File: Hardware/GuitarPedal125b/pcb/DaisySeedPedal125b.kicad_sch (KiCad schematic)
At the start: 6 parts, among them J1 Barrel_Jack_Switch, J2 AUDIO_IN_TRS, J3 AUDIO_OUT_TRS, J4 MIDI IN JACK, J5 MIDI OUT JACK

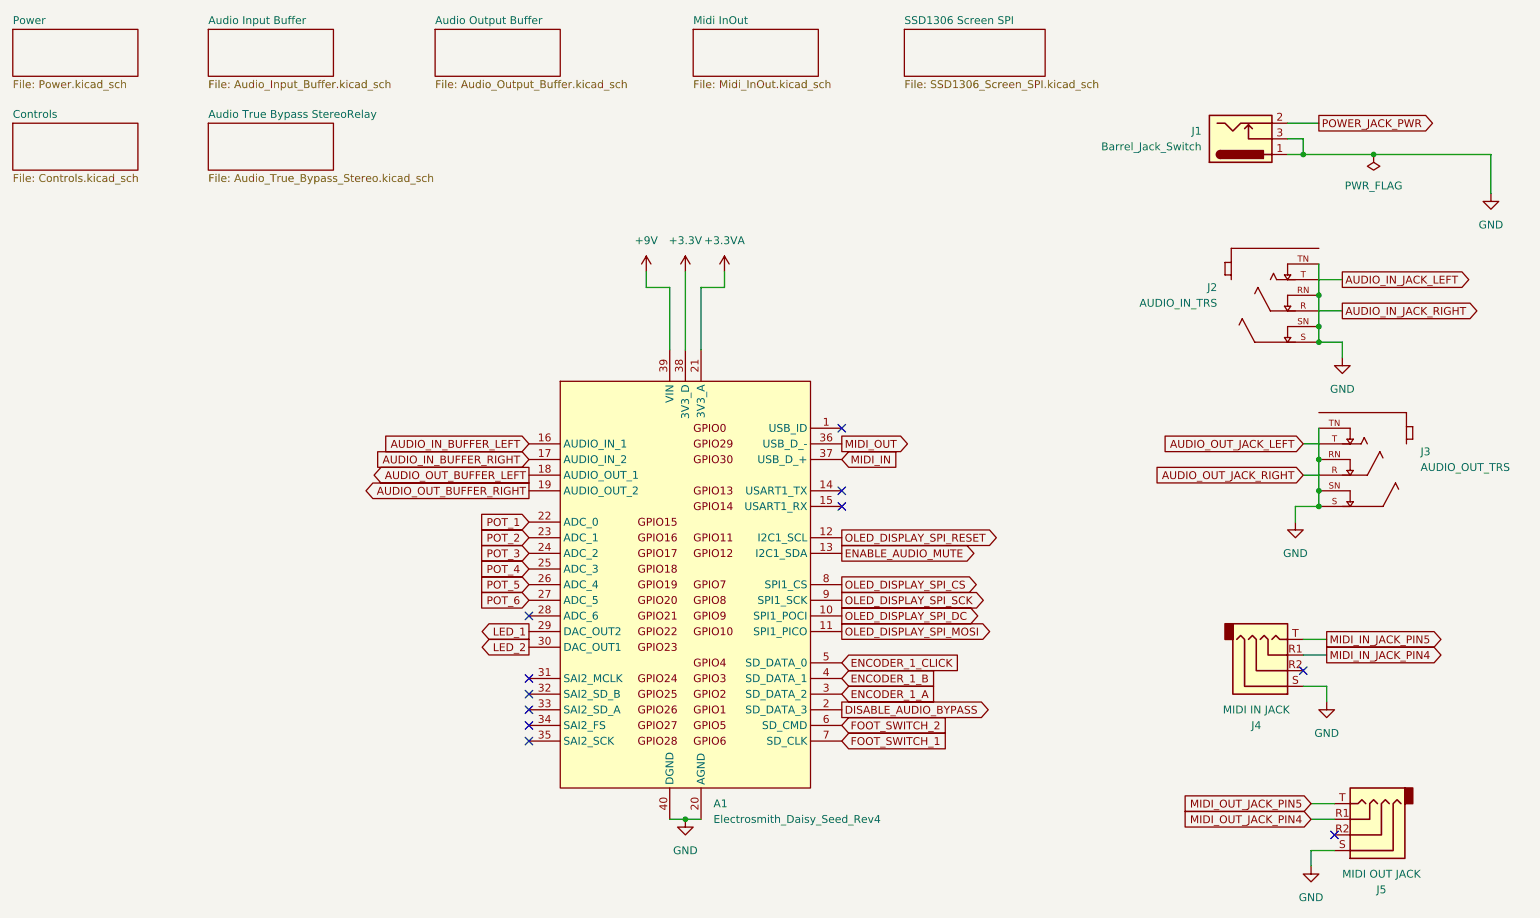
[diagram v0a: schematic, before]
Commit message: Rev6 WIP
Working on a fresh layout of the board.
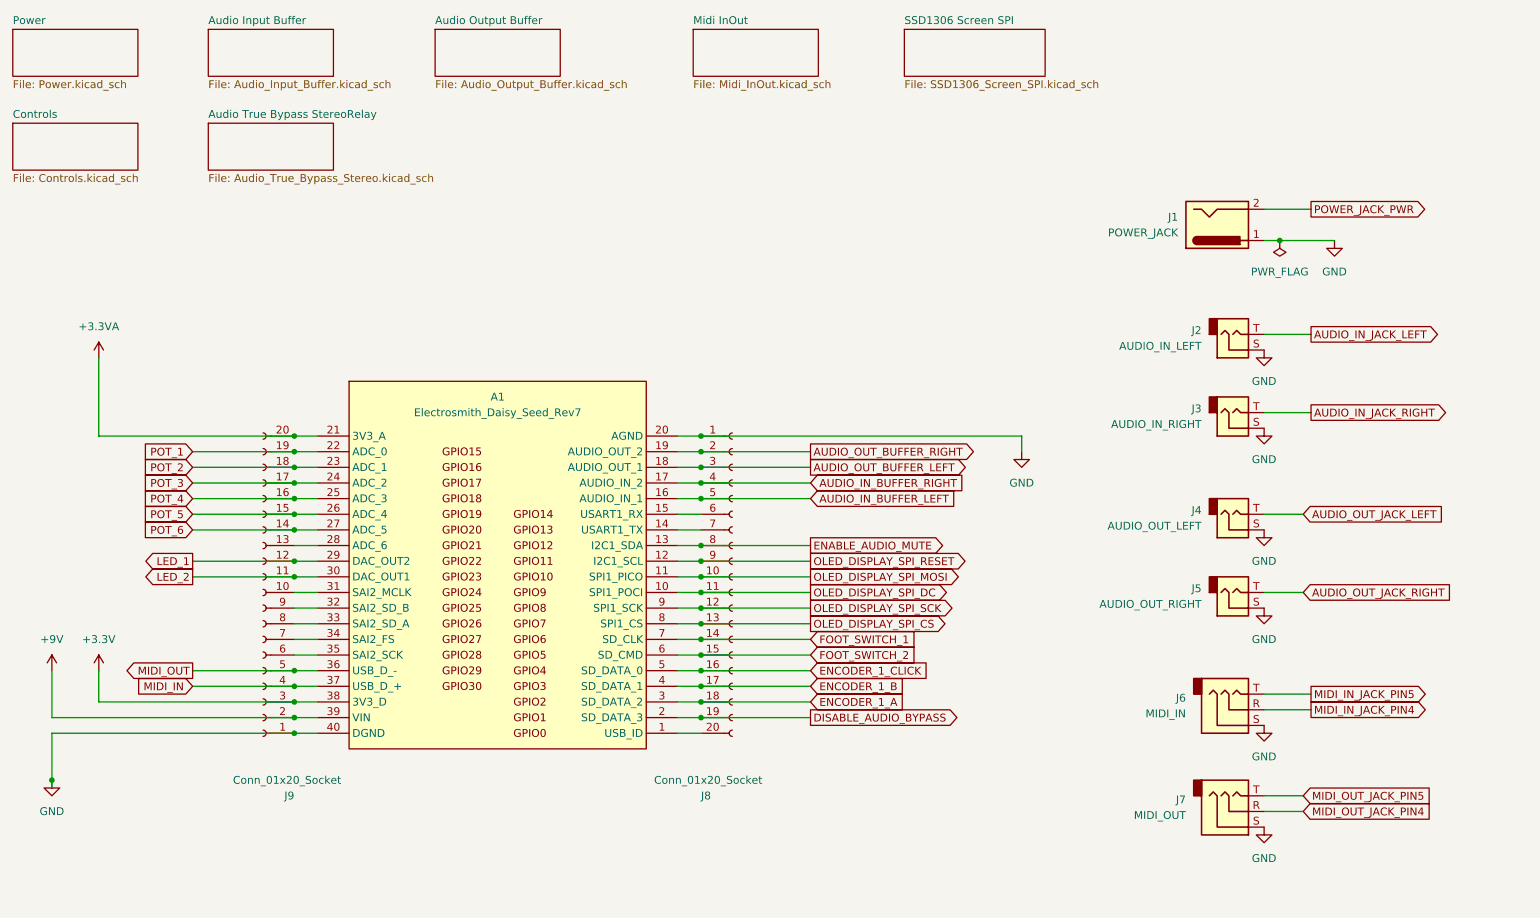
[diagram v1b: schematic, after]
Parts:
- removed J3: AUDIO_OUT_TRS, NMJ6HCD2:NEUTRIK_NMJ6HCD2, symbol NMJ6HCD2:NMJ6HCD2
- removed J5: MIDI OUT JACK, AudioConnector-PJ320A:TRRS-PJ-320A, symbol Connector_Audio:AudioJack4
- added J3: AUDIO_IN_RIGHT, GuitarPedal125B:Generic_Pads_AudioTS, symbol Connector_Audio:AudioJack2
- added J4: AUDIO_OUT_LEFT, GuitarPedal125B:Generic_Pads_AudioTS, symbol Connector_Audio:AudioJack2
- added J5: AUDIO_OUT_RIGHT, GuitarPedal125B:Generic_Pads_AudioTS, symbol Connector_Audio:AudioJack2
- added J7: MIDI_OUT, GuitarPedal125B:Generic_Pads_AudioTRS, symbol Connector_Audio:AudioJack3
- added J8, J9: Conn_01x20_Socket, Connector_PinSocket_2.54mm:PinSocket_1x20_P2.54mm_Vertical, symbol Connector:Conn_01x20_Socket
- A1: value Electrosmith_Daisy_Seed_Rev4 -> Electrosmith_Daisy_Seed_Rev7; footprint Module:Electrosmith_Daisy_Seed -> (none); symbol MCU_Module:Electrosmith_Daisy_Seed_Rev4 -> GuitarPedal125B:Electrosmith_Daisy_Seed_Rev7; now left out of the parts list
- J1: value Barrel_Jack_Switch -> POWER_JACK; footprint GuitarPedal125B:Generic_PowerJack -> GuitarPedal125B:Generic_Pads_Power; symbol Connector:Barrel_Jack_Switch -> Connector:Barrel_Jack
- J2: value AUDIO_IN_TRS -> AUDIO_IN_LEFT; footprint NMJ6HCD2:NEUTRIK_NMJ6HCD2 -> GuitarPedal125B:Generic_Pads_AudioTS; symbol NMJ6HCD2:NMJ6HCD2 -> Connector_Audio:AudioJack2
- J6: renamed from J4; value MIDI IN JACK -> MIDI_IN; footprint AudioConnector-PJ320A:TRRS-PJ-320A -> GuitarPedal125B:Generic_Pads_AudioTRS; symbol Connector_Audio:AudioJack4 -> Connector_Audio:AudioJack3
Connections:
- net +3.3V: now also J9.3 (Pin_3)
- net +3.3VA: now also J9.20 (Pin_20)
- net +9V: now also J9.2 (Pin_2)
- net AUDIO_IN_BUFFER_LEFT: now also J8.5 (Pin_5)
- net AUDIO_IN_BUFFER_RIGHT: now also J8.4 (Pin_4)
- net AUDIO_IN_JACK_RIGHT: now also J3.T; no longer J2.R
- net AUDIO_OUT_BUFFER_LEFT: now also J8.3 (Pin_3)
- net AUDIO_OUT_BUFFER_RIGHT: now also J8.2 (Pin_2)
- net AUDIO_OUT_JACK_LEFT: now also J4.T
- net AUDIO_OUT_JACK_RIGHT: now also J5.T
- net DISABLE_AUDIO_BYPASS: now also J8.19 (Pin_19)
- net ENABLE_AUDIO_MUTE: now also J8.8 (Pin_8)
- net ENCODER_1_A: now also J8.18 (Pin_18)
- net ENCODER_1_B: now also J8.17 (Pin_17)
- net ENCODER_1_CLICK: now also J8.16 (Pin_16)
- net FOOT_SWITCH_1: now also J8.14 (Pin_14)
- net FOOT_SWITCH_2: now also J8.15 (Pin_15)
- net GND: now also J3.S, J4.S, J5.S, J7.S, J8.1 (Pin_1), J9.1 (Pin_1); no longer J1.3, J2.RN, J2.SN, J2.TN
- net LED_1: now also J9.12 (Pin_12)
- net LED_2: now also J9.11 (Pin_11)
- net MIDI_IN: now also J9.4 (Pin_4)
- net MIDI_IN_JACK_PIN4: now also J6.R; no longer J6.R1
- net MIDI_OUT: now also J9.5 (Pin_5)
- net MIDI_OUT_JACK_PIN4: now also J7.R
- net MIDI_OUT_JACK_PIN5: now also J7.T
- net OLED_DISPLAY_SPI_CS: now also J8.13 (Pin_13)
- net OLED_DISPLAY_SPI_DC: now also J8.11 (Pin_11)
- net OLED_DISPLAY_SPI_MOSI: now also J8.10 (Pin_10)
- net OLED_DISPLAY_SPI_RESET: now also J8.9 (Pin_9)
- net OLED_DISPLAY_SPI_SCK: now also J8.12 (Pin_12)
- net POT_1: now also J9.19 (Pin_19)
- net POT_2: now also J9.18 (Pin_18)
- net POT_3: now also J9.17 (Pin_17)
- net POT_4: now also J9.16 (Pin_16)
- net POT_5: now also J9.15 (Pin_15)
- net POT_6: now also J9.14 (Pin_14)
- net at A1.1 (USB_ID): now also J8.20 (Pin_20)
- net at A1.14 (USART1_TX): now also J8.7 (Pin_7)
- net at A1.15 (USART1_RX): now also J8.6 (Pin_6)
- net at A1.28 (ADC_6): now also J9.13 (Pin_13)
- net at A1.31 (SAI2_MCLK): now also J9.10 (Pin_10)
- net at A1.32 (SAI2_SD_B): now also J9.9 (Pin_9)
- net at A1.33 (SAI2_SD_A): now also J9.8 (Pin_8)
- net at A1.34 (SAI2_FS): now also J9.7 (Pin_7)
- net at A1.35 (SAI2_SCK): now also J9.6 (Pin_6)
- no-connect marks 11 -> 0
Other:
- moved on the sheet: A1
